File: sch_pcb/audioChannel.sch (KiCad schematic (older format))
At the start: 81 parts, among them J204 DE9F, Q201 BSS138, Q202 BSS138, Q203 BSS138, U103 MCP4351, U201 MCP6004N, U202 74LVC1G3157, U203 74LVC1G3157, U204 74LVC4066, U205 MCP6004N, U206 74LVC1G3157, U207 MCP6S26

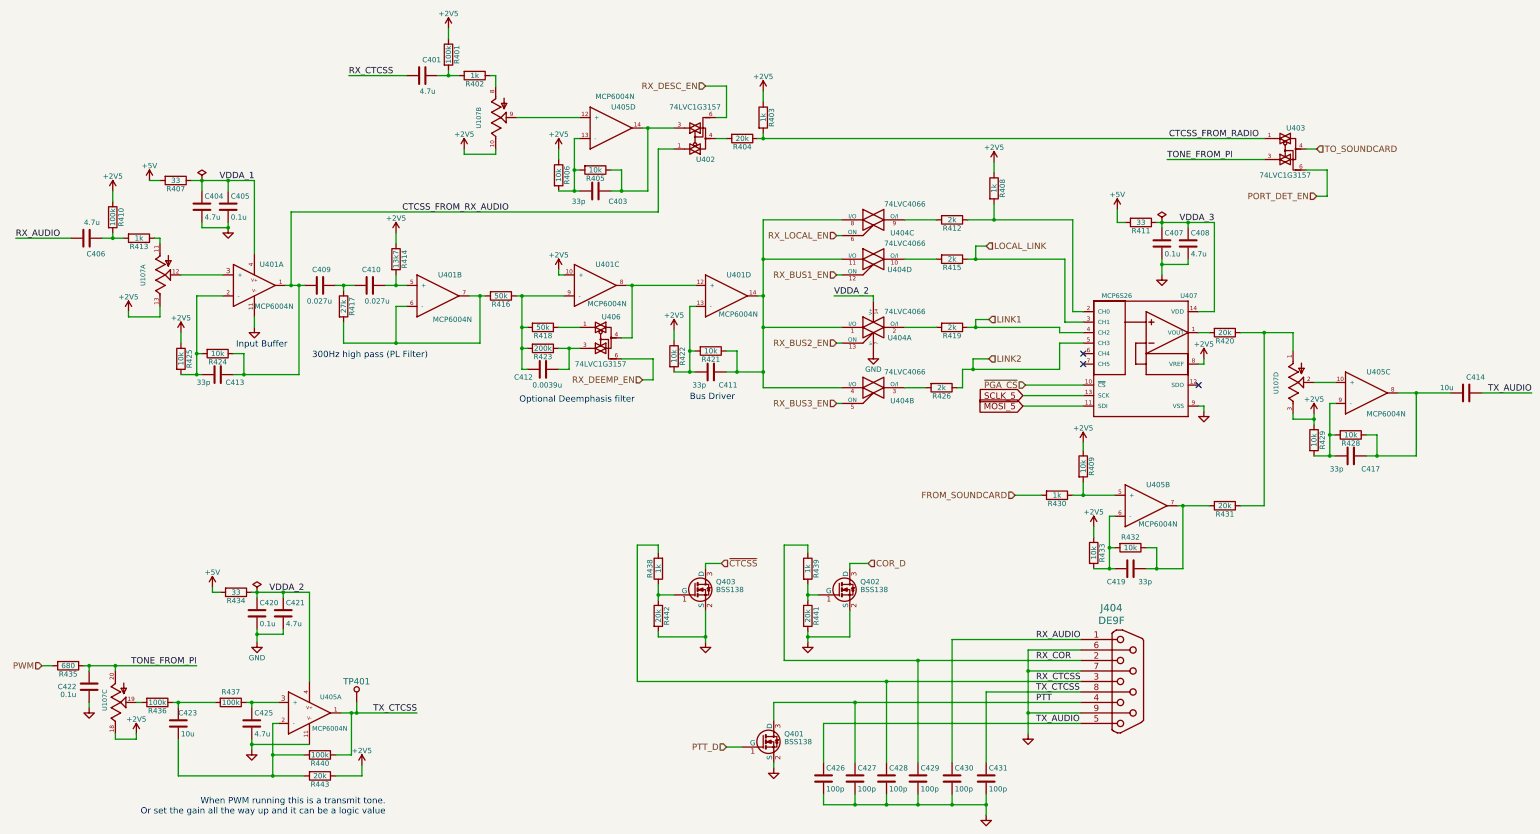
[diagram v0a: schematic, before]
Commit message: Add files via upload
Remove OLED connector
Remove extra bypass cap from third EEPOT
More routing - got the soundcards and usb hub done.  Only remaining big section is the DC-DC.  Still a bit of pain-in-the-tuchas traces that need to sneak across the board...
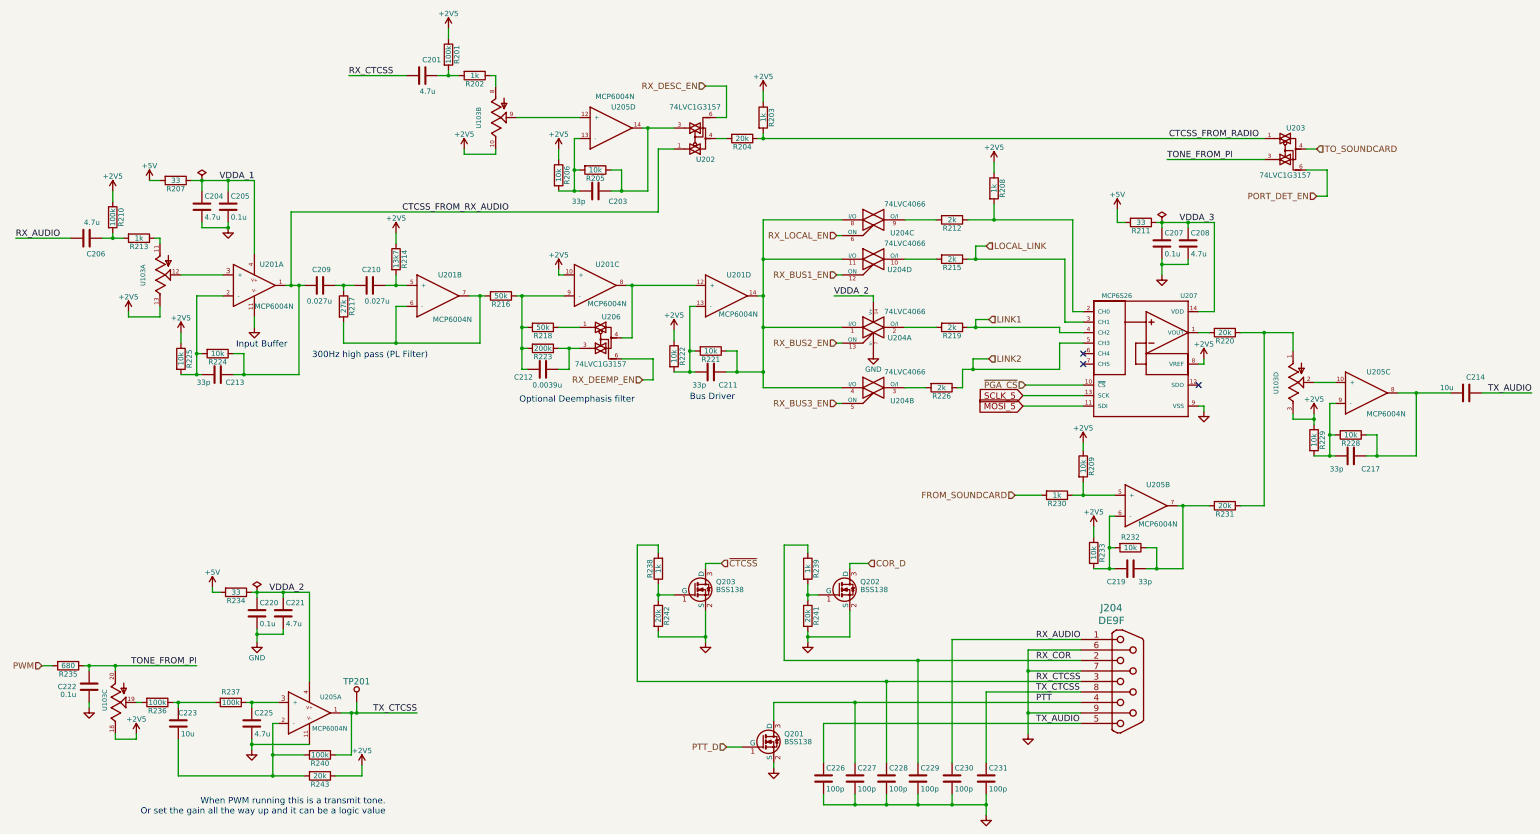
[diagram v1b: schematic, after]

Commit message: Add files via upload
Fix sheet ordering in schematic
Finish routing (except USB connector...)
Still to do: USB connector, cleanup PCB, fix refdes positions
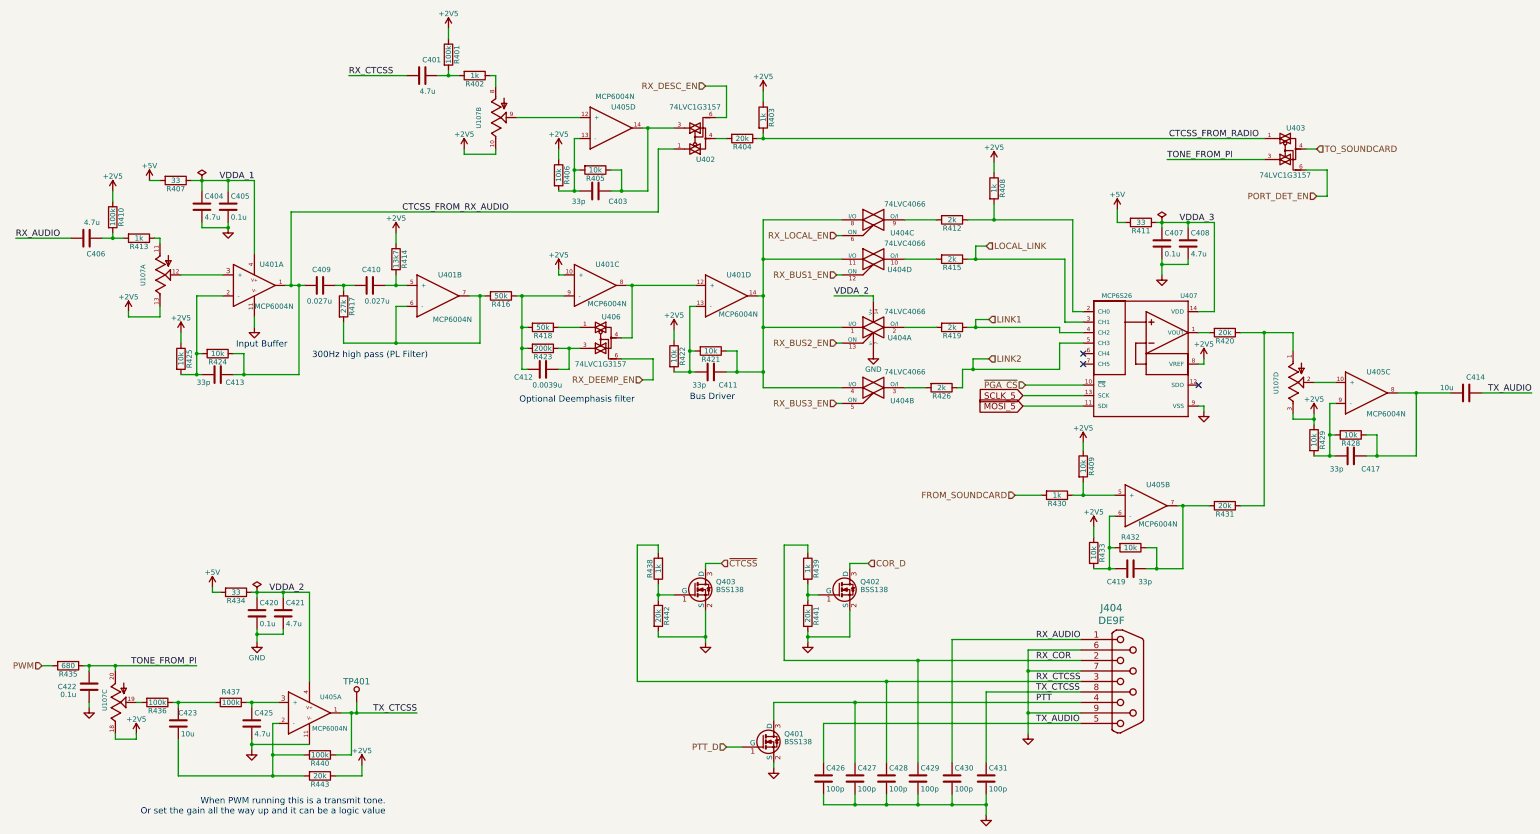
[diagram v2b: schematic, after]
